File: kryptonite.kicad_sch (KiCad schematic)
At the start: 28 parts, among them J1 Conn_01x04_Pin, P2 USB_C_Plug, SW1 SW_Push, SW2 SW_Push, U1 STM32F072CBUx, U2 ATECC608B-MAHDA, U3 MCP1700x-330xxTT, U4 USBLC6-2SC6, Y1 8MHz

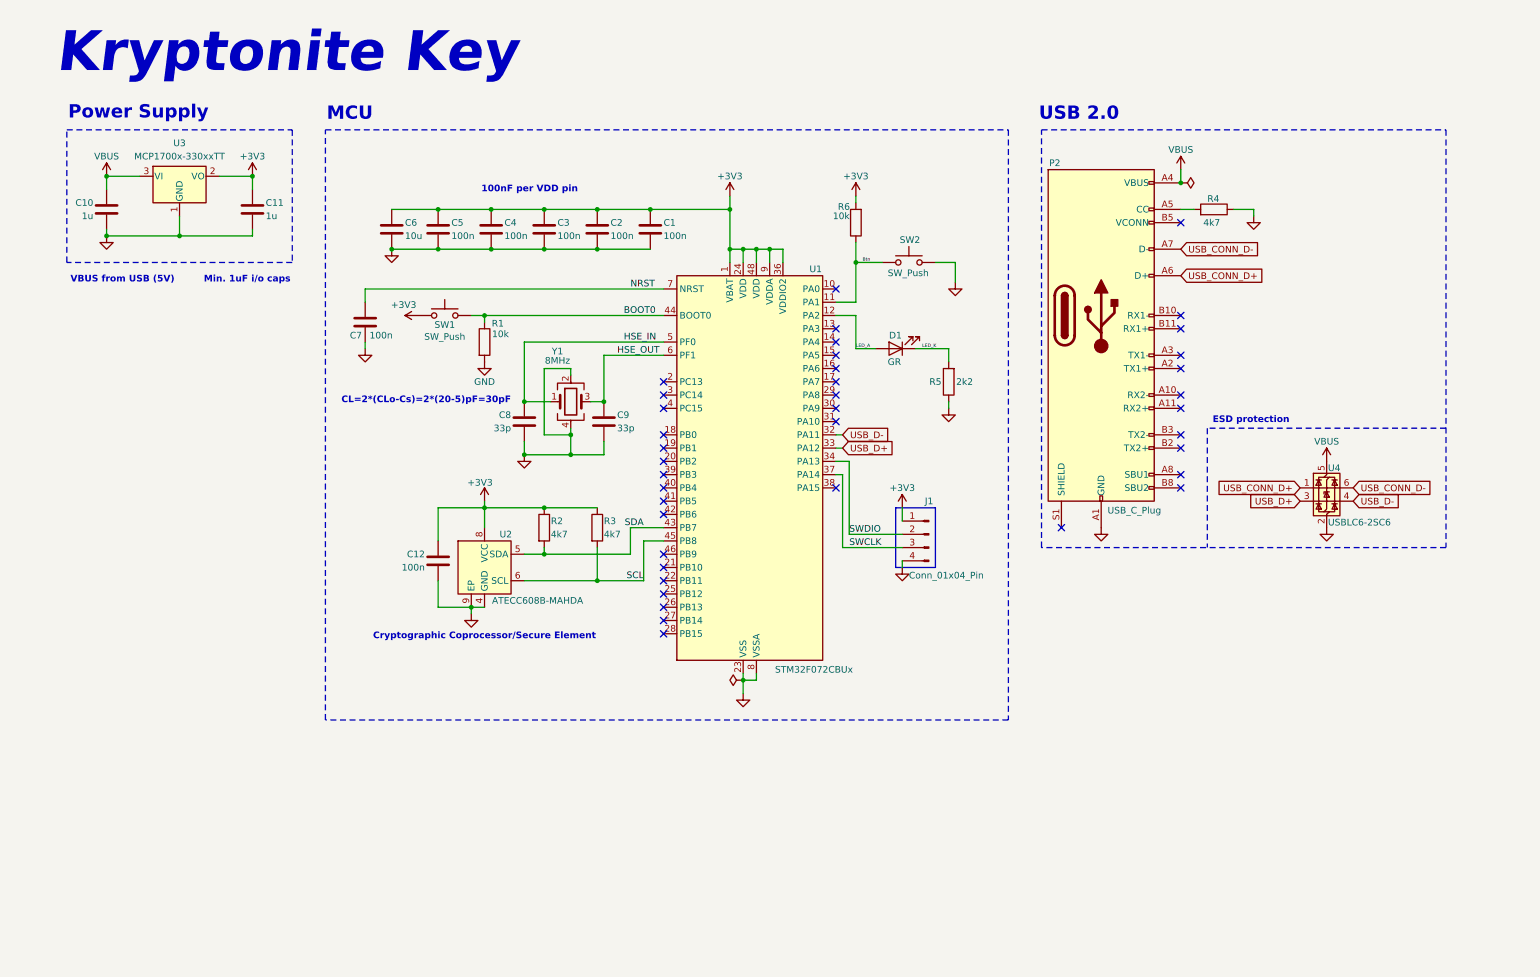
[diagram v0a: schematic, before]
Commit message: did some stuff
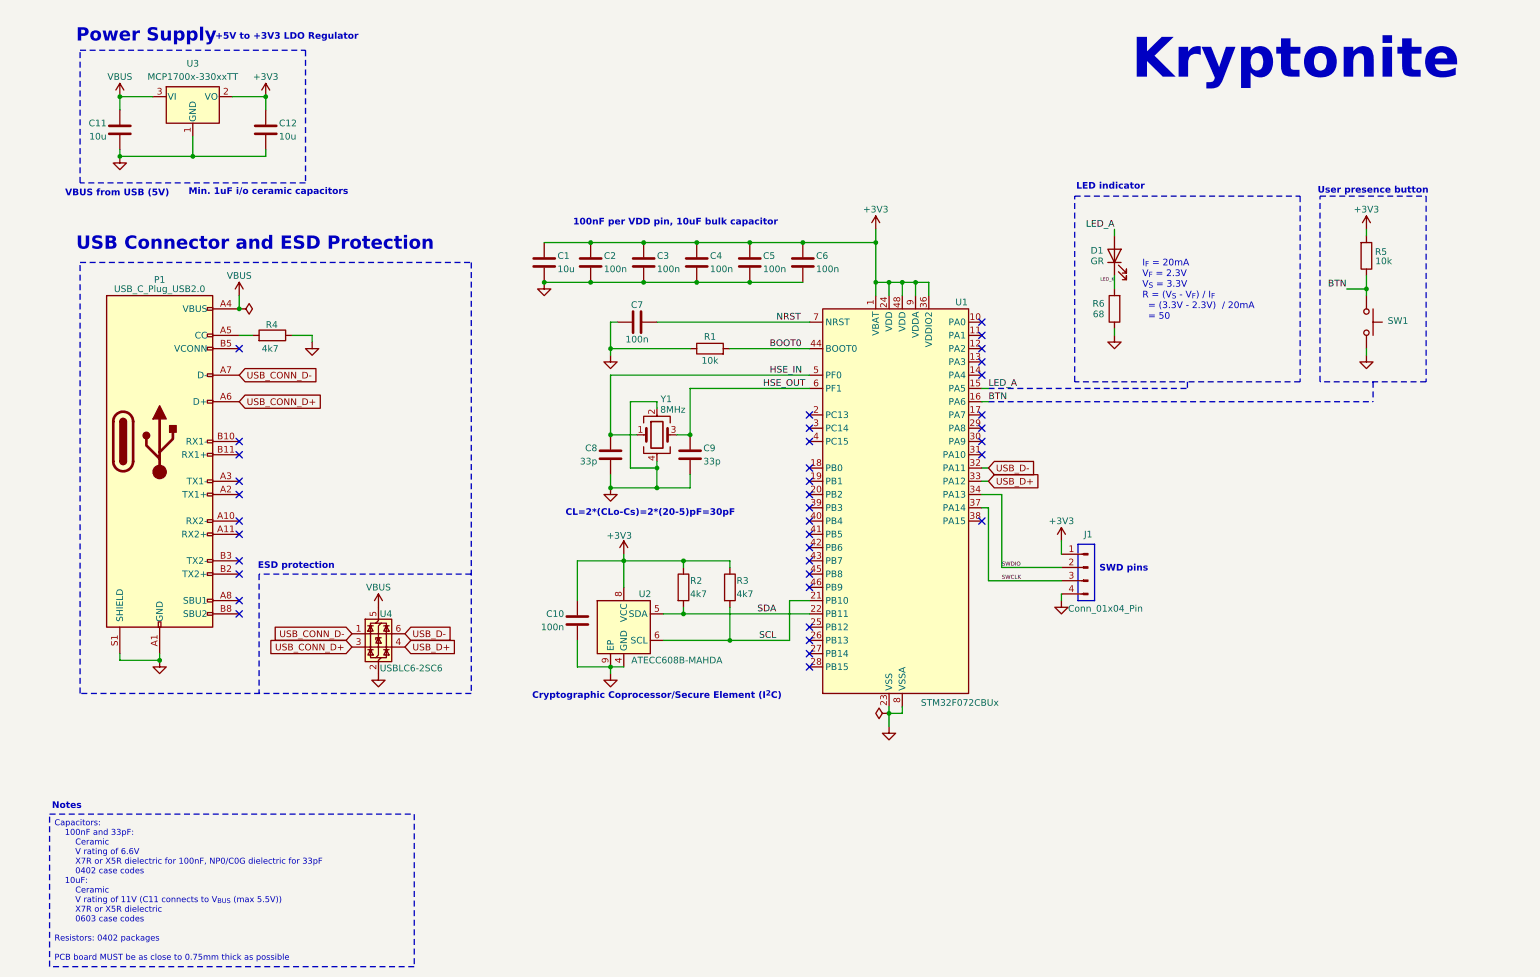
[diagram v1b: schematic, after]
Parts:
- removed P2: USB_C_Plug, symbol Connector:USB_C_Plug
- removed SW1: SW_Push, Button_Switch_SMD:SW_Push_1P1T_XKB_TS-1187A, symbol Switch:SW_Push
- added P1: USB_C_Plug_USB2.0, type-c:TYPE-C-31-G-01, symbol Connector:USB_C_Plug
- C1: renamed from C6; footprint Capacitor_SMD:C_0805_2012Metric_Pad1.18x1.45mm_HandSolder -> Capacitor_SMD:C_0603_1608Metric
- C10: renamed from C12; footprint Capacitor_SMD:C_0402_1005Metric_Pad0.74x0.62mm_HandSolder -> Capacitor_SMD:C_0402_1005Metric
- C11: renamed from C10; value 1u -> 10u; footprint Capacitor_SMD:C_0805_2012Metric_Pad1.18x1.45mm_HandSolder -> Capacitor_SMD:C_0603_1608Metric
- C12: renamed from C11; value 1u -> 10u; footprint Capacitor_SMD:C_0805_2012Metric_Pad1.18x1.45mm_HandSolder -> Capacitor_SMD:C_0603_1608Metric
- C2: renamed from C5; footprint Capacitor_SMD:C_0402_1005Metric_Pad0.74x0.62mm_HandSolder -> Capacitor_SMD:C_0402_1005Metric
- C3: renamed from C4; footprint Capacitor_SMD:C_0402_1005Metric_Pad0.74x0.62mm_HandSolder -> Capacitor_SMD:C_0402_1005Metric
- C4: renamed from C3; footprint Capacitor_SMD:C_0402_1005Metric_Pad0.74x0.62mm_HandSolder -> Capacitor_SMD:C_0402_1005Metric
- C5: renamed from C2; footprint Capacitor_SMD:C_0402_1005Metric_Pad0.74x0.62mm_HandSolder -> Capacitor_SMD:C_0402_1005Metric
- C6: renamed from C1; footprint Capacitor_SMD:C_0402_1005Metric_Pad0.74x0.62mm_HandSolder -> Capacitor_SMD:C_0402_1005Metric
- C7, C8, C9: footprint Capacitor_SMD:C_0402_1005Metric_Pad0.74x0.62mm_HandSolder -> Capacitor_SMD:C_0402_1005Metric
- D1: Distributer Link (none) -> https://www.lcsc.com/product-detail/Light-Emitting-Diodes-L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; Manufacturer (none) -> XINGLIGHT; Manufacturer Part Number (none) -> XL-1608SURC-06
- J1: Distributer Link (none) -> https://www.lcsc.com/product-detail/Pin-Headers_CONNFLY-Ele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; Manufacturer (none) -> CONNFLY; Manufacturer Part Number (none) -> DS1021-1x4SF11-B
- R1: footprint Resistor_SMD:R_0402_1005Metric_Pad0.72x0.64mm_HandSolder -> Resistor_SMD:R_0402_1005Metric; Distributer Link (none) -> https://www.lcsc.com/product-detail/Chip-Resistor-Surface-M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; Manufacturer (none) -> YAGEO; Manufacturer Part Number (none) -> RC0402FR-0710KL
- R2, R3, R4: footprint Resistor_SMD:R_0402_1005Metric_Pad0.72x0.64mm_HandSolder -> Resistor_SMD:R_0402_1005Metric; Distributer Link (none) -> https://www.lcsc.com/product-detail/Chip-Resistor-Surface-M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; Manufacturer (none) -> UNI-ROYAL(Uniroyal Elec); Manufacturer Part Number (none) -> 0402WGJ0472TCE
- R5: renamed from R6; footprint Resistor_SMD:R_0402_1005Metric_Pad0.72x0.64mm_HandSolder -> Resistor_SMD:R_0402_1005Metric; Distributer Link (none) -> https://www.lcsc.com/product-detail/Chip-Resistor-Surface-M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; Manufacturer (none) -> YAGEO; Manufacturer Part Number (none) -> RC0402FR-0710KL
- R6: renamed from R5; value 2k2 -> 68; footprint Resistor_SMD:R_0402_1005Metric_Pad0.72x0.64mm_HandSolder -> Resistor_SMD:R_0402_1005Metric; Distributer Link (none) -> https://www.lcsc.com/product-detail/Chip-Resistor-Surface-M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; Manufacturer (none) -> FOJAN; Manufacturer Part Number (none) -> FRC0402J680 TS
- SW1: renamed from SW2; Distributer Link (none) -> https://www.lcsc.com/product-detail/Tactile-Switches_XKB-Co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; Manufacturer (none) -> XKB Connection; Manufacturer Part Number (none) -> TS-1187A-B-A-B
- U1: Distributer Link (none) -> https://www.lcsc.com/product-detail/Microcontrollers-MCU-MP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; Manufacturer (none) -> STMicroelectronics; Manufacturer Part Number (none) -> STM32F072CBU6
- U2: Distributer Link (none) -> https://www.lcsc.com/product-detail/Security-Verification-E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; Manufacturer (none) -> Microchip Tech; Manufacturer Part Number (none) -> ATECC608B-MAHDA-S
- U3: Distributer Link (none) -> https://www.lcsc.com/product-detail/Voltage-Regulators-Line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; Manufacturer (none) -> Microchip Tech; Manufacturer Part Number (none) -> MCP1700T-3302E/TT
- U4: Distributer Link (none) -> https://www.lcsc.com/product-detail/ESD-and-Surge-Protectio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; Manufacturer (none) -> STMicroelectronics; Manufacturer Part Number (none) -> USBLC6-2SC6
- Y1: Distributer Link (none) -> https://www.lcsc.com/product-detail/Crystals_Yajingxin-TAXM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; Manufacturer (none) -> Yajingxin; Manufacturer Part Number (none) -> TAXM8M4RLBDDT2T
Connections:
- net BOOT0: now also R1.2; no longer R1.1
- net GND: now also R1.1, P1.A1 (GND), P1.A12 (GND), P1.B1 (GND), P1.B12 (GND), P1.S1 (SHIELD); no longer R1.2
- net LED_A: now also U1.15 (PA5); no longer U1.12 (PA2)
- net SCL: now also U1.21 (PB10); no longer U1.45 (PB8)
- net SDA: now also U1.22 (PB11); no longer U1.43 (PB7)
- net USB_CONN_D+: now also U4.3 (I/O2), P1.A6 (D+); no longer U4.1 (I/O1)
- net USB_CONN_D-: now also U4.1 (I/O1), P1.A7 (D-); no longer U4.6 (I/O1)
- net USB_D+: now also U4.4 (I/O2); no longer U4.3 (I/O2)
- net USB_D-: now also U4.6 (I/O1); no longer U4.4 (I/O2)
- net VBUS: now also P1.A4 (VBUS), P1.A9 (VBUS), P1.B4 (VBUS), P1.B9 (VBUS)
- net at R4.2: now also P1.A5 (CC)
- net BTN: now reaches U1.16 (PA6)
- net BTN: now also R5.1, SW1.1
- removed net Btn: R5.1, SW1.1, U1.11 (PA1)
- no-connect marks 39 -> 38
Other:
- note added: "+5V to +3V3 LDO Regulator"
- note added: "100nF per VDD pin, 10uF bulk capacitor"
- note added: "Cryptographic Coprocessor/Secure Element (I^{2}C)"
- note added: "I_{F} = 20mA V_{F} = 2.3V V_{S} = 3.3V R = (V_{S} - V_{F}) / I_{F} = (3.3V - 2.3V) / 20mA = 50"
- note added: "Kryptonite"
- note added: "LED indicator"
- note added: "Min. 1uF i/o ceramic capacitors"
- note added: "Notes"
- note added: "SWD pins"
- note added: "USB Connector and ESD Protection"
- note added: "User presence button"
- note removed: "100nF per VDD pin"
- note removed: "Cryptographic Coprocessor/Secure Element"
- note removed: "Kryptonite Key"
- note removed: "MCU"
- note removed: "Min. 1uF i/o caps"
- note removed: "USB 2.0"
- title: Kryptonite Key -> Kryptonite
- moved on the sheet: C1, C10, C11, C12, C2, C3, C4, C5, C6, C7, C8, C9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
